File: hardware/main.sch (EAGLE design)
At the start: 89 parts, among them IC1 MPU-6050, IC2 TB6612FNG, Q1 TEFT4300, Q2 TEFT4300, Q3 TEFT4300, Q4 TEFT4300, Q5 TEFT4300, Q6 TEFT4300, Q7 IRLML2244, Q8 8MHz, T1 IRLML0030, T2 IRLML0030, T3 IRLML0030, T4 IRLML0030, T5 IRLML0030, T6 IRLML0030, T8 IRLML0030

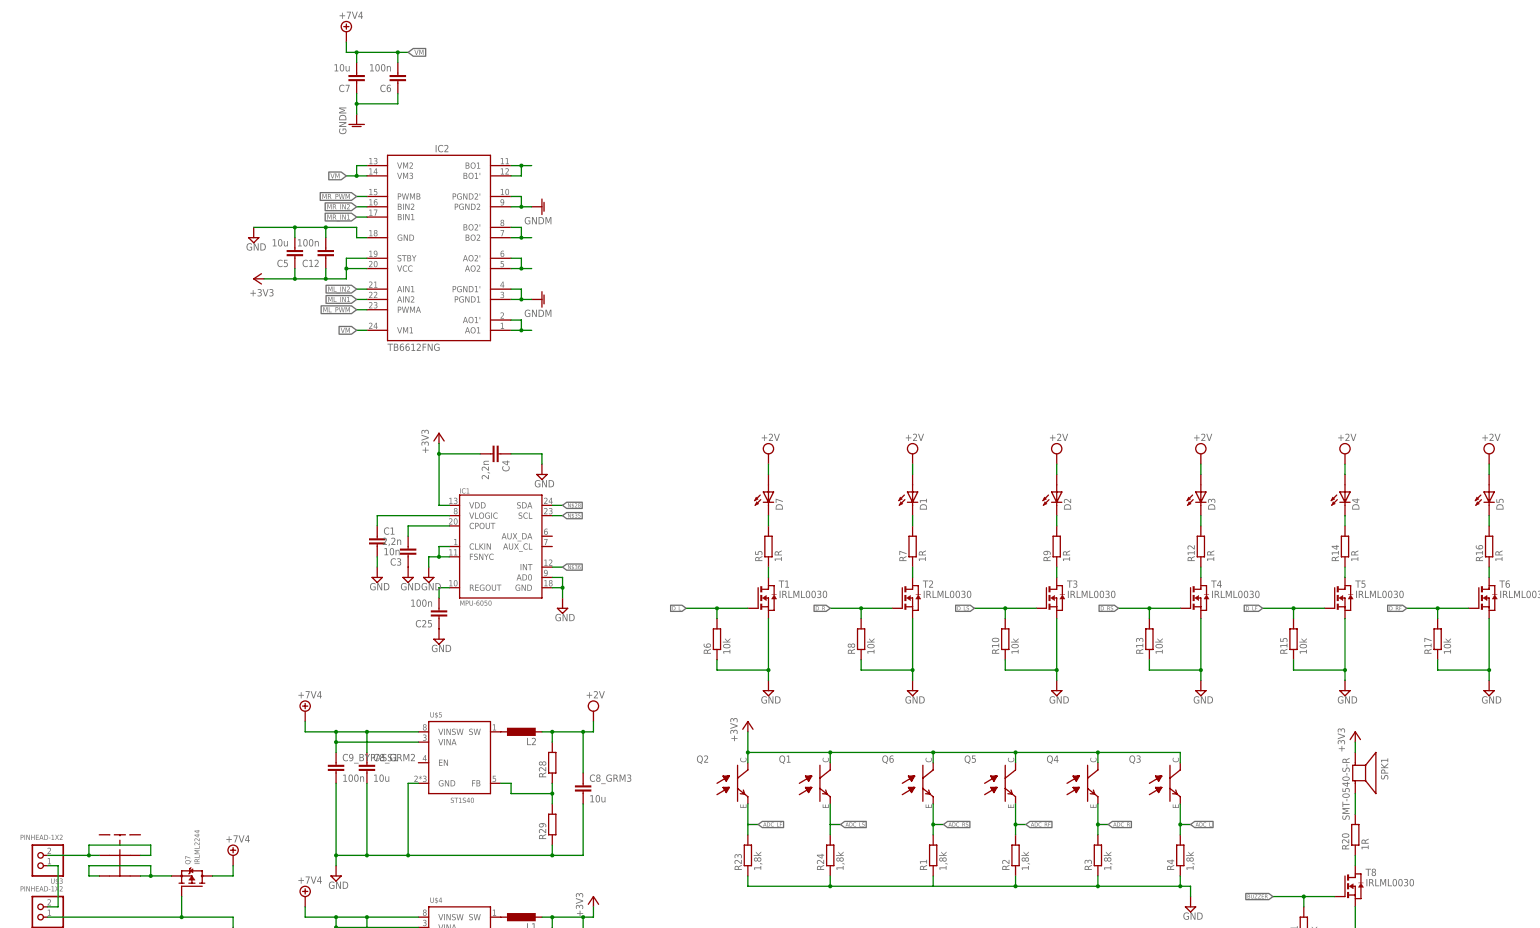
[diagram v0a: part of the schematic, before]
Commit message: encoder brd
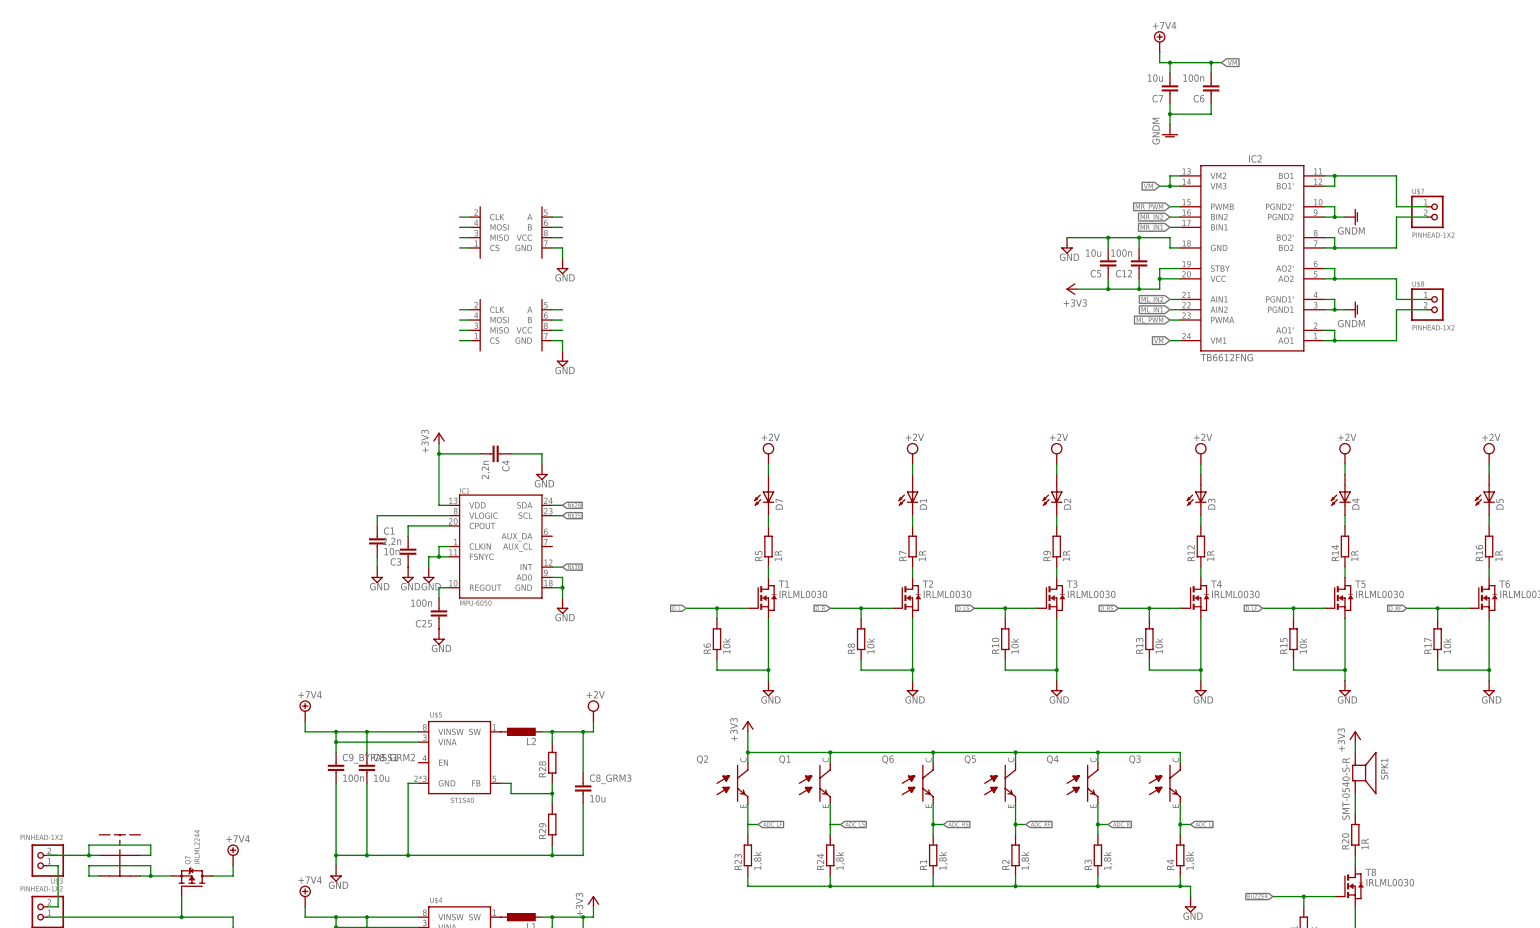
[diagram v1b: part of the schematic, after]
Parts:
- added U$10, U$9: ENCODER_MOUNT, micromouse:ENCODER_MOUNT
- added U$7, U$8: PINHEAD-1X2, BaseApp:PINHEAD-1X2
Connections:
- new net N$14: U$9.CLK
- new net N$15: U$9.MOSI
- new net N$16: U$9.MISO
- new net N$17: U$9.CS
- new net N$18: U$9.A
- new net N$19: U$9.B
- new net N$20: U$9.VCC
- new net N$22: U$10.A
- new net N$24: U$10.B
- new net N$25: U$10.VCC
- new net N$32: U$10.CS
- new net N$42: U$10.MISO
- new net N$44: U$10.MOSI
- new net N$45: U$10.CLK
- net GND: now also U$10.GND, U$9.GND
- net N$37: now also U$8.2
- net N$38: now also U$7.1
- net N$39: now also U$7.2
- net N$40: now also U$8.1
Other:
- moved on the sheet: C12, C5, C6, C7, IC2
